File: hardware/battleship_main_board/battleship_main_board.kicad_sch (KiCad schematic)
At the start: 5 parts

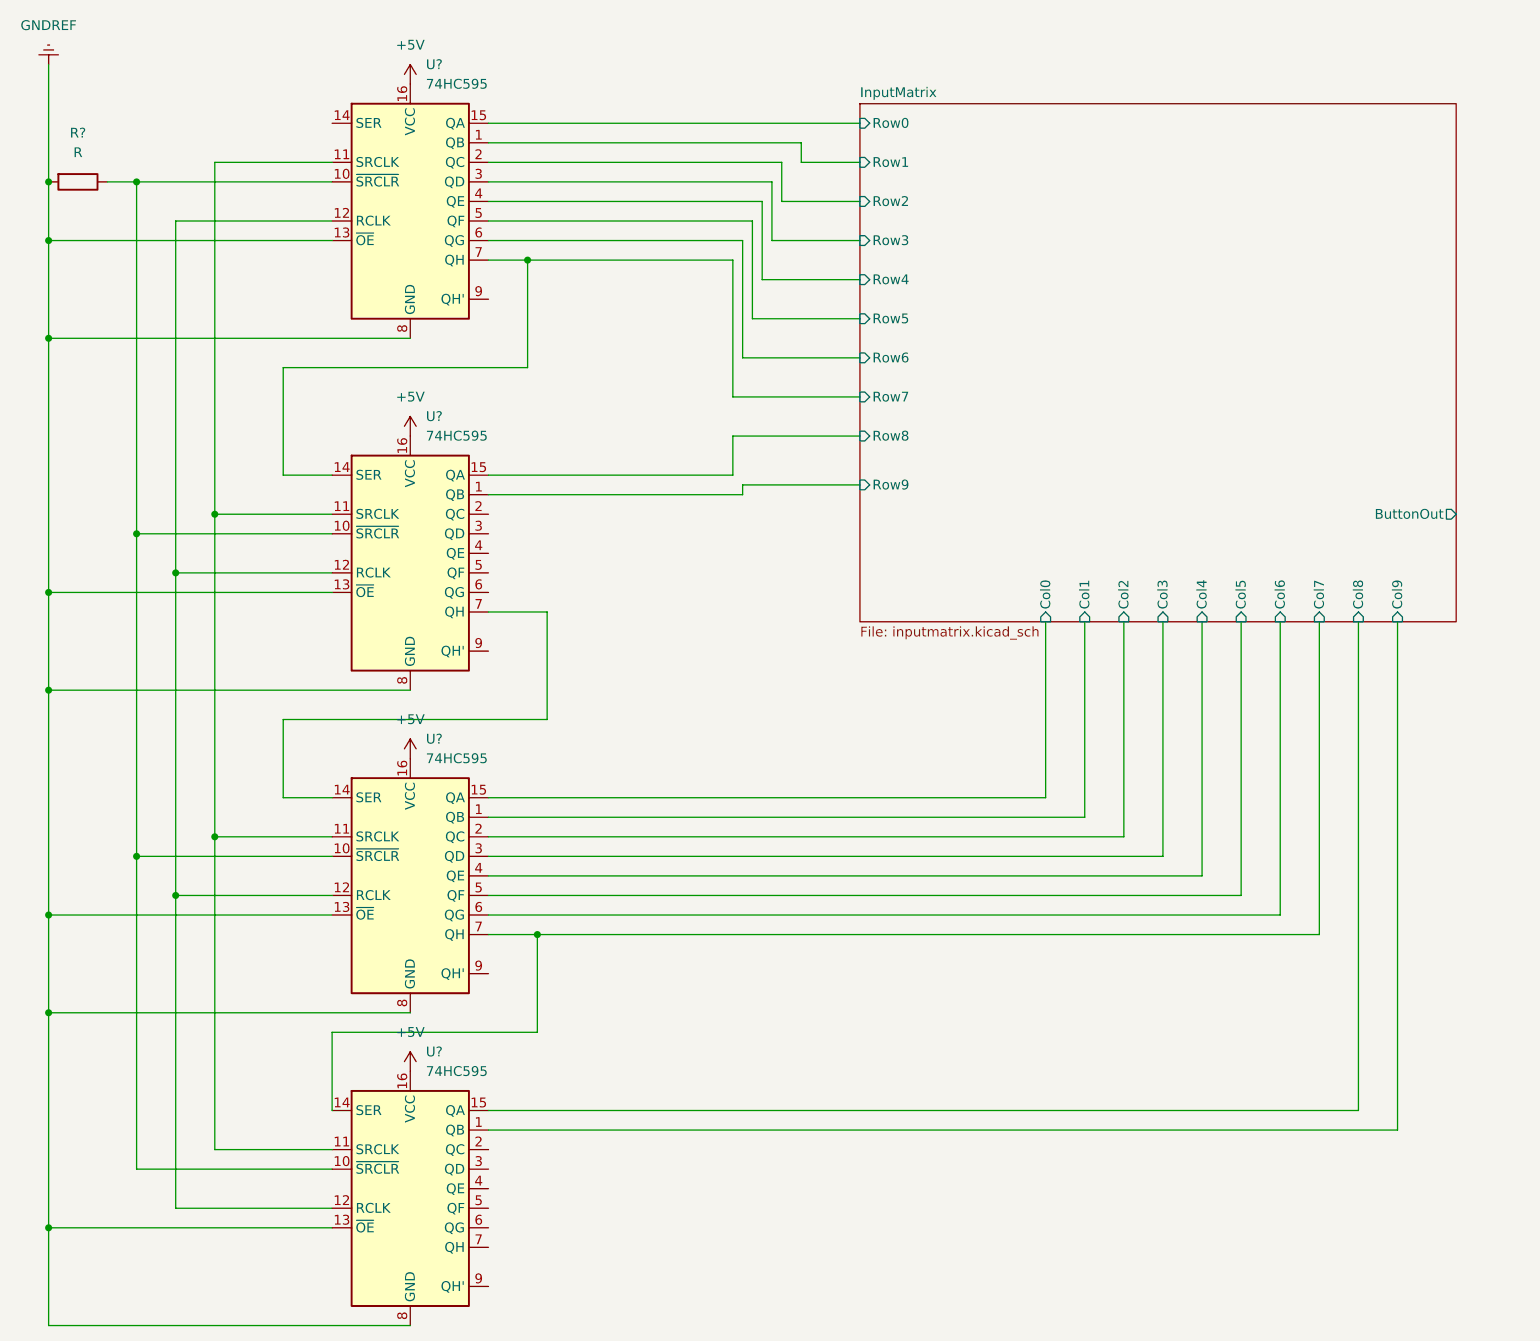
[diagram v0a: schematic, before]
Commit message: Work on main board
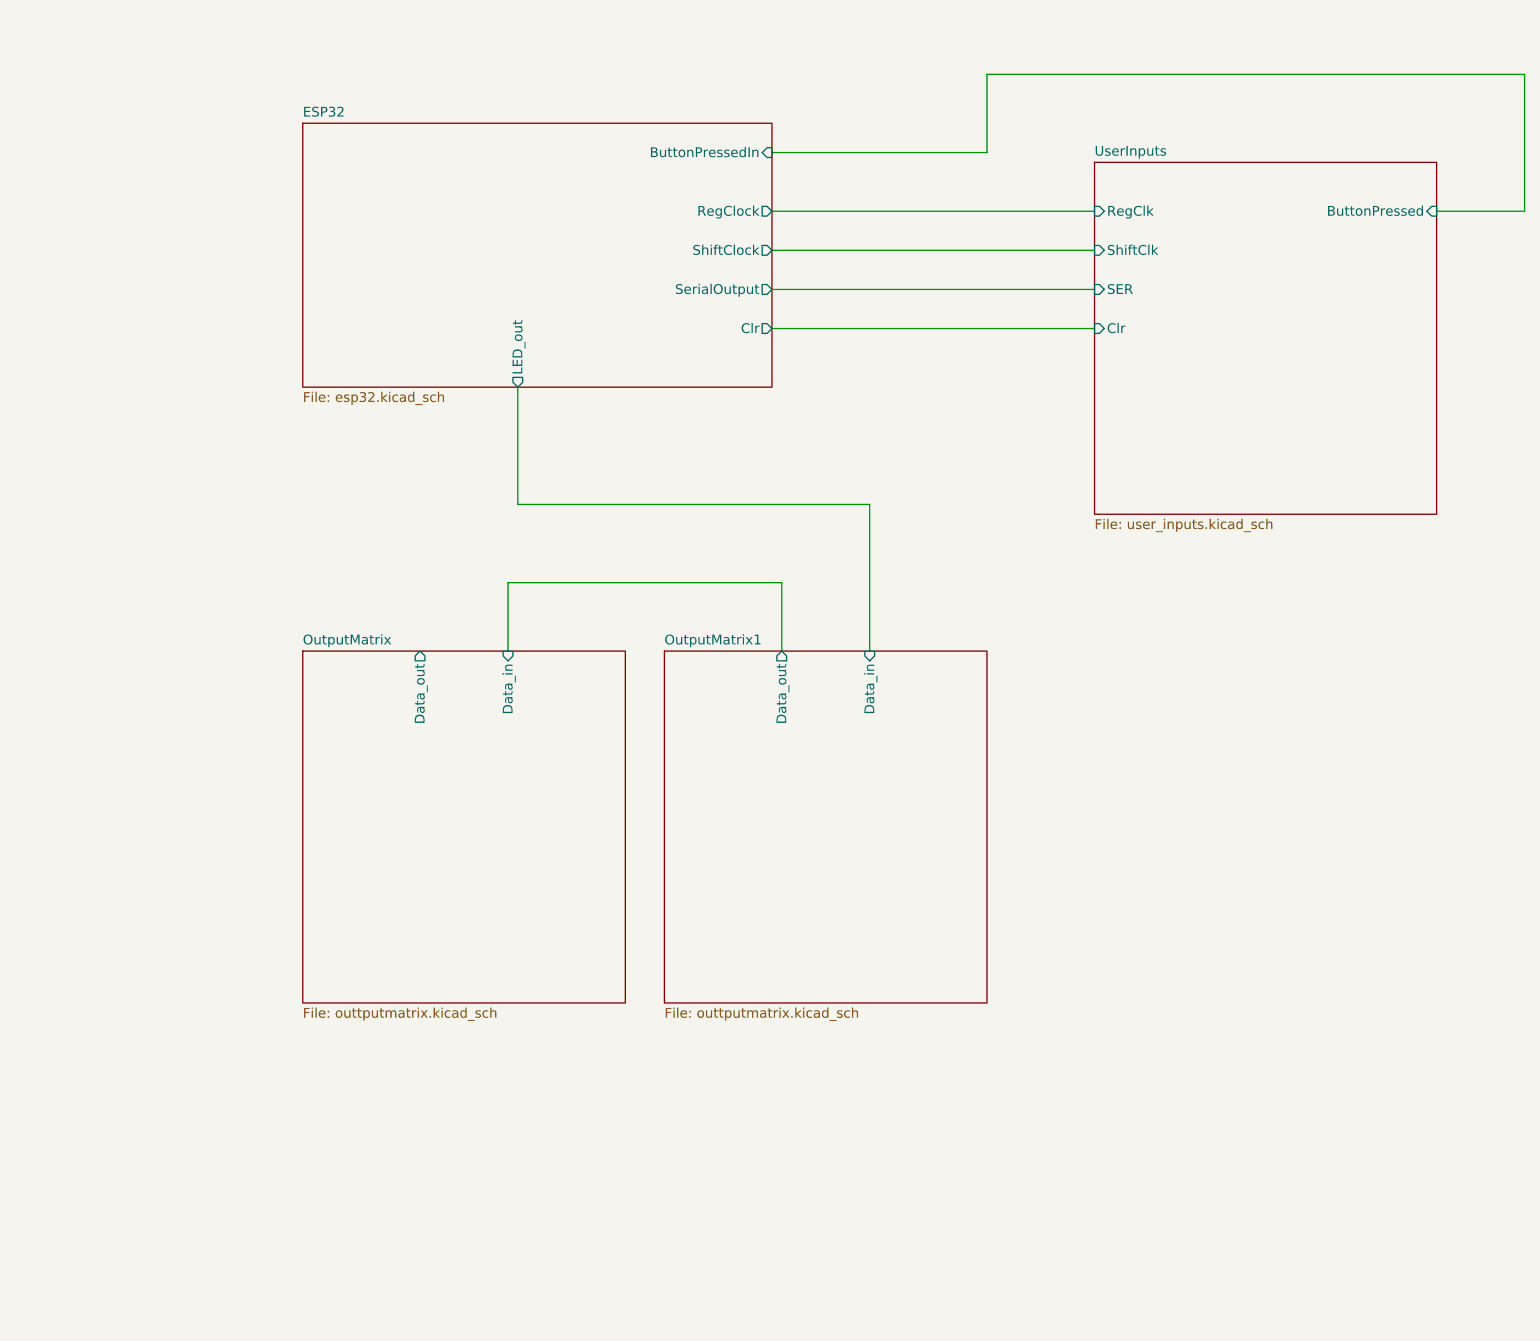
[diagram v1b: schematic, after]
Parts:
- removed R?: R, symbol Device:R
- removed U? (x4): 74HC595, symbol 74xx:74HC595
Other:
- removed sheet InputMatrix
- added sheet ESP32 (esp32.kicad_sch)
- added sheet OutputMatrix (outtputmatrix.kicad_sch)
- added sheet OutputMatrix1 (outtputmatrix.kicad_sch)
- added sheet UserInputs (user_inputs.kicad_sch)
